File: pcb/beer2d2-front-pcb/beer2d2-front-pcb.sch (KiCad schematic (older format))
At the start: 8 parts, among them IC1 ATTINY167, IC2 LM1117, J1 6-12V, P1 AVR_ISP

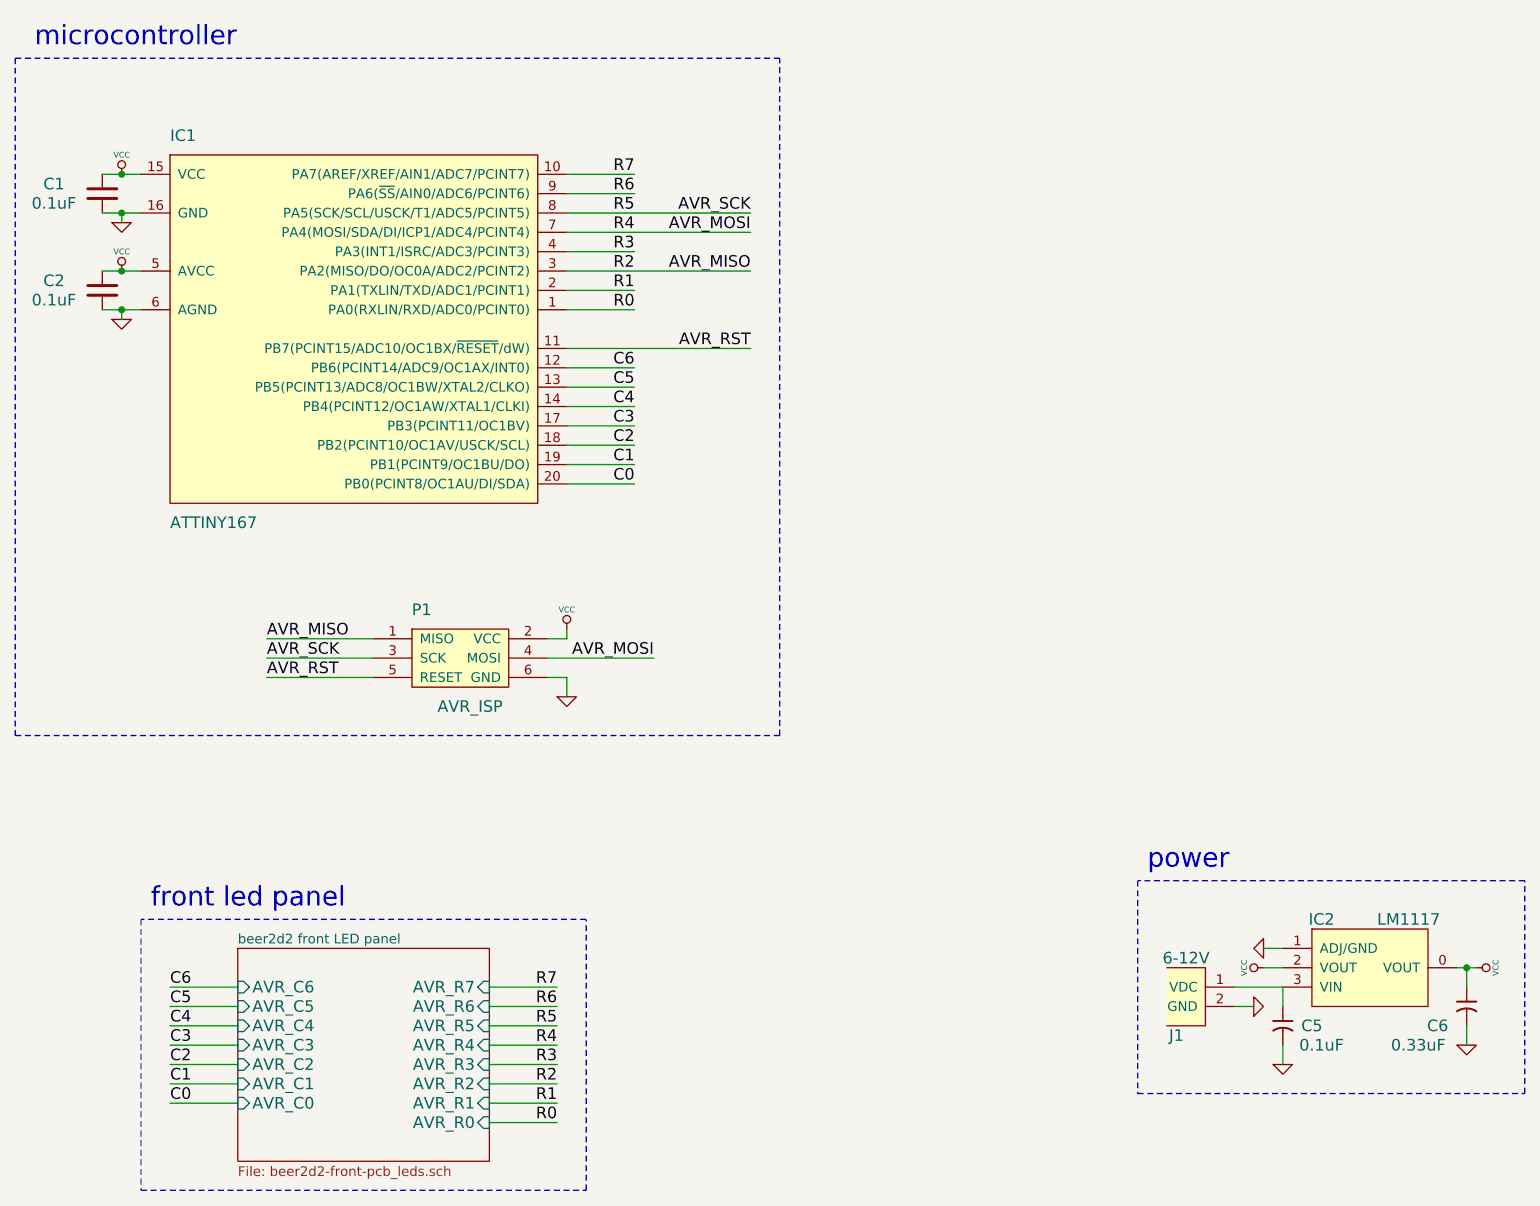
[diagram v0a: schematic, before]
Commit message: moving on to rear pcb
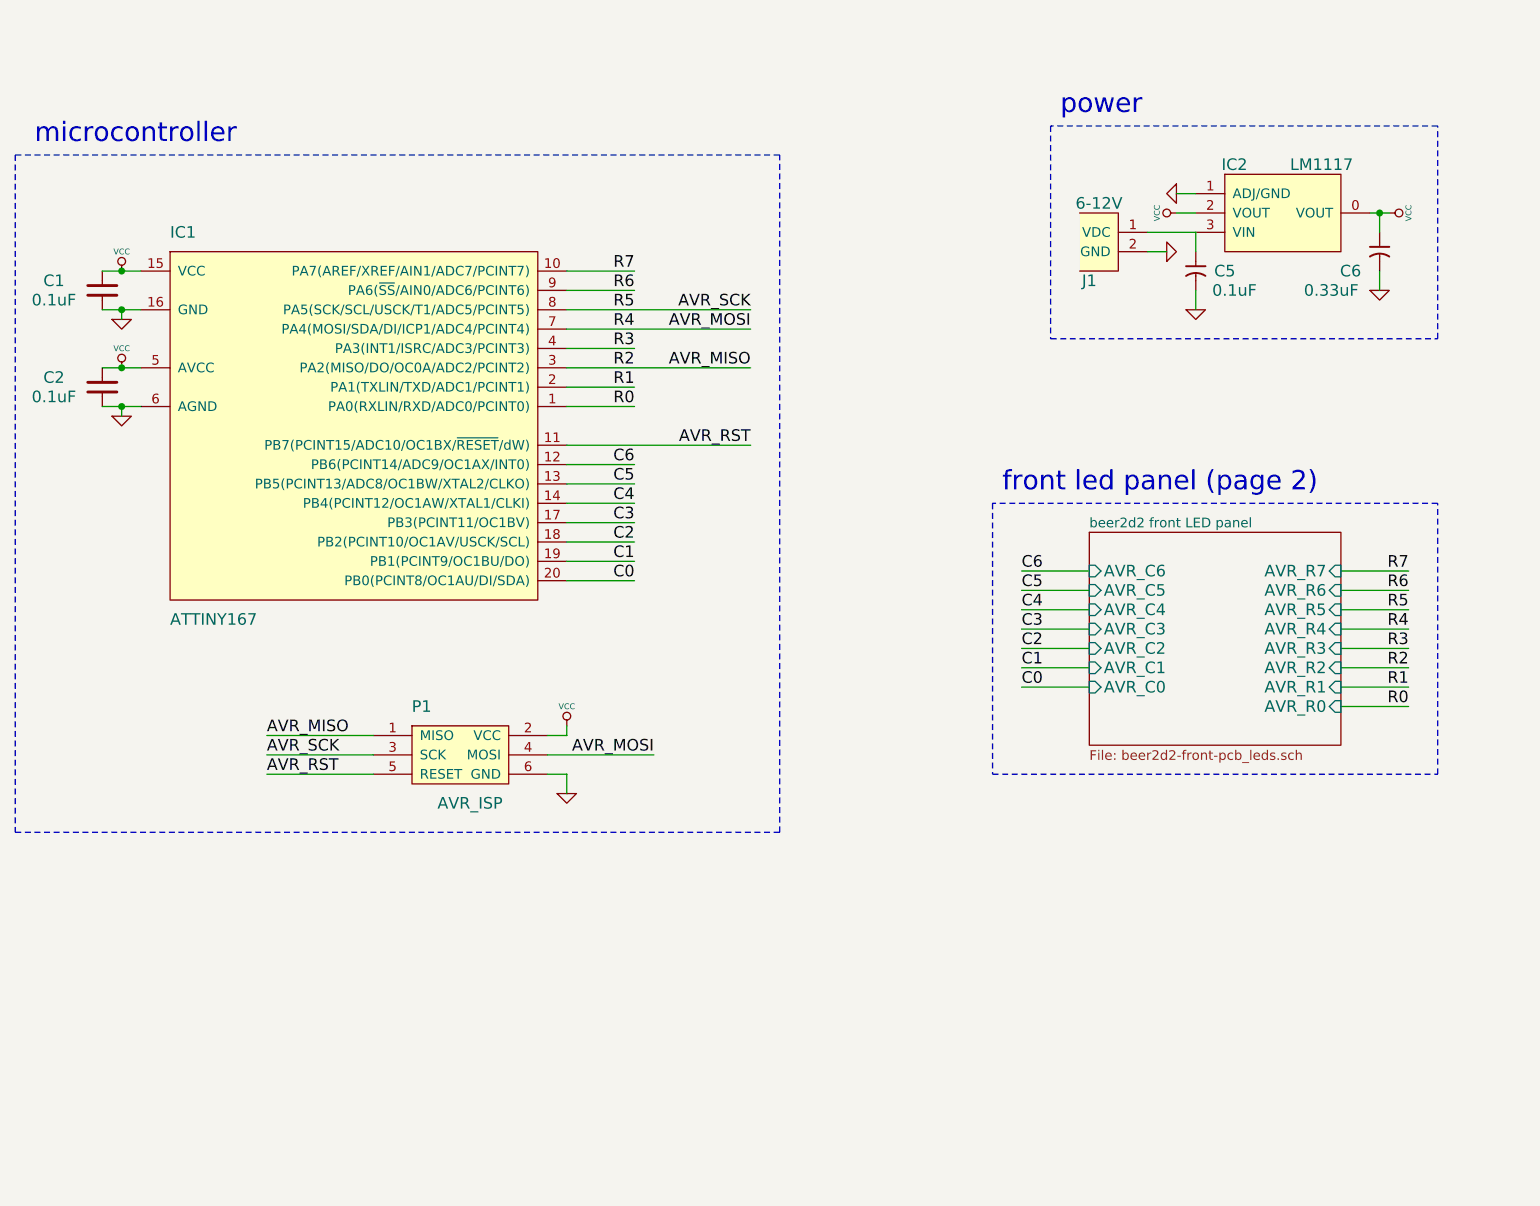
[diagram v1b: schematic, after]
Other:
- note added: "front led panel (page 2)"
- note removed: "front led panel"
- moved on the sheet: C1, C2, C5, C6, IC1, IC2, J1, P1
